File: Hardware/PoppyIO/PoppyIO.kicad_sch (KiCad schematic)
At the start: 0 parts

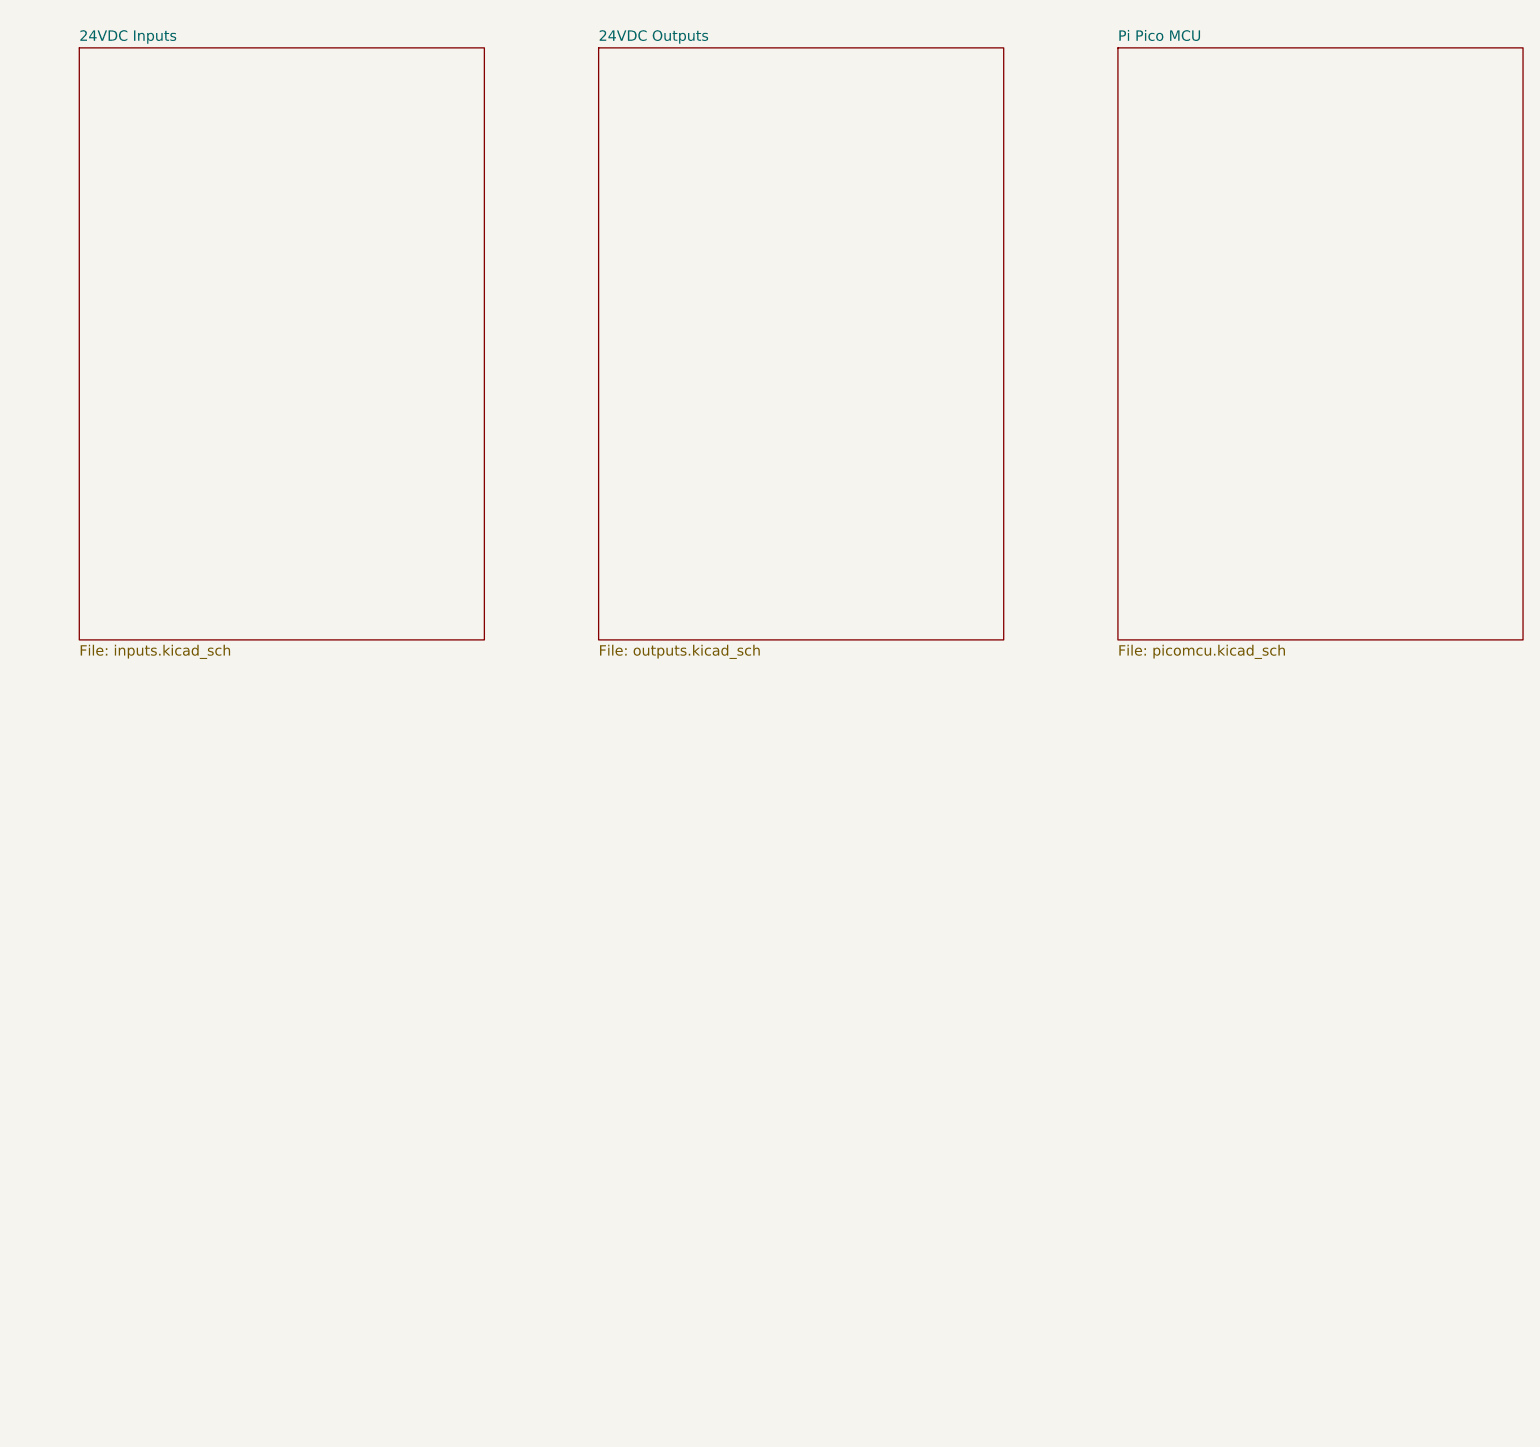
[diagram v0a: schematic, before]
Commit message: hw: io: Updates
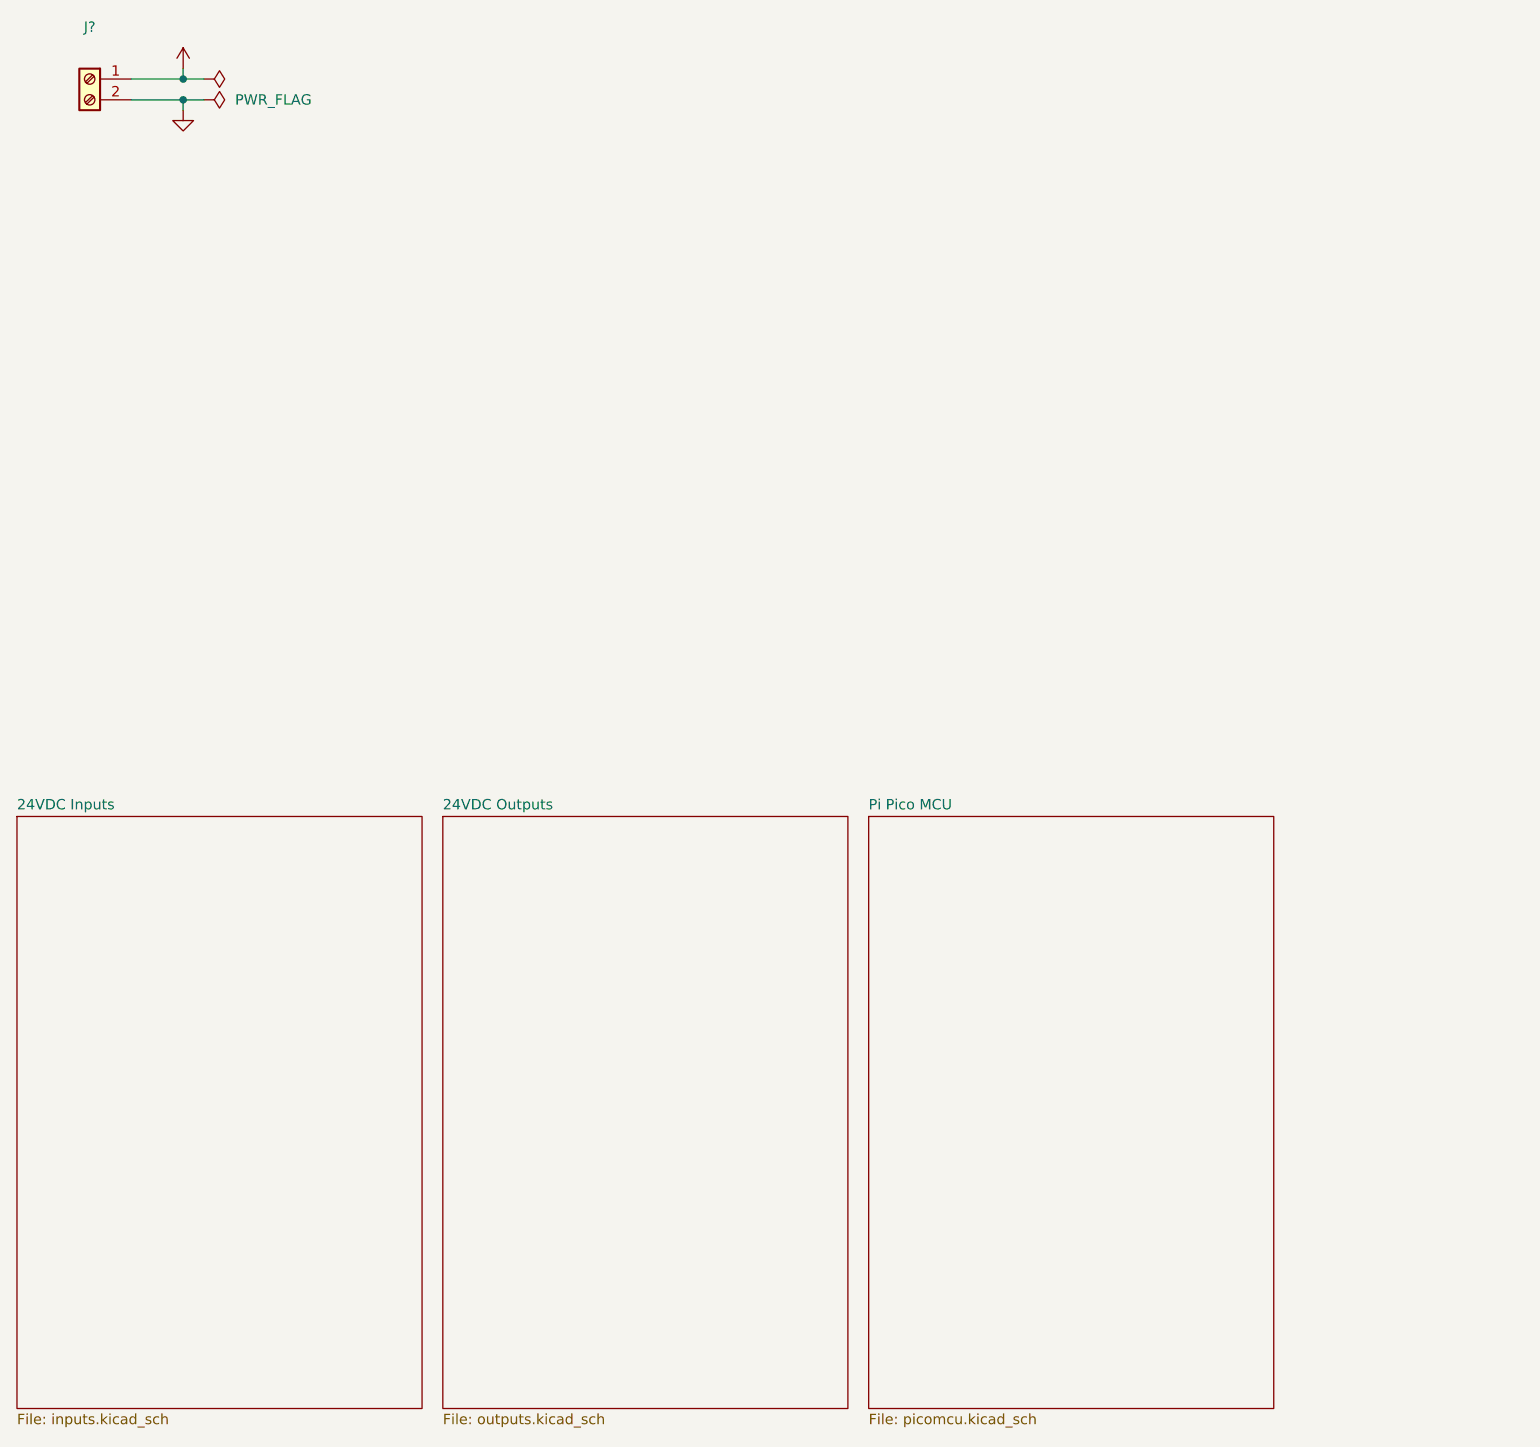
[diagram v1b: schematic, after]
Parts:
- added J?: (no value), symbol Connector:Screw_Terminal_01x02
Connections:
- new net +5V: J?.1 (Pin_1)
- new net GND: J?.2 (Pin_2)

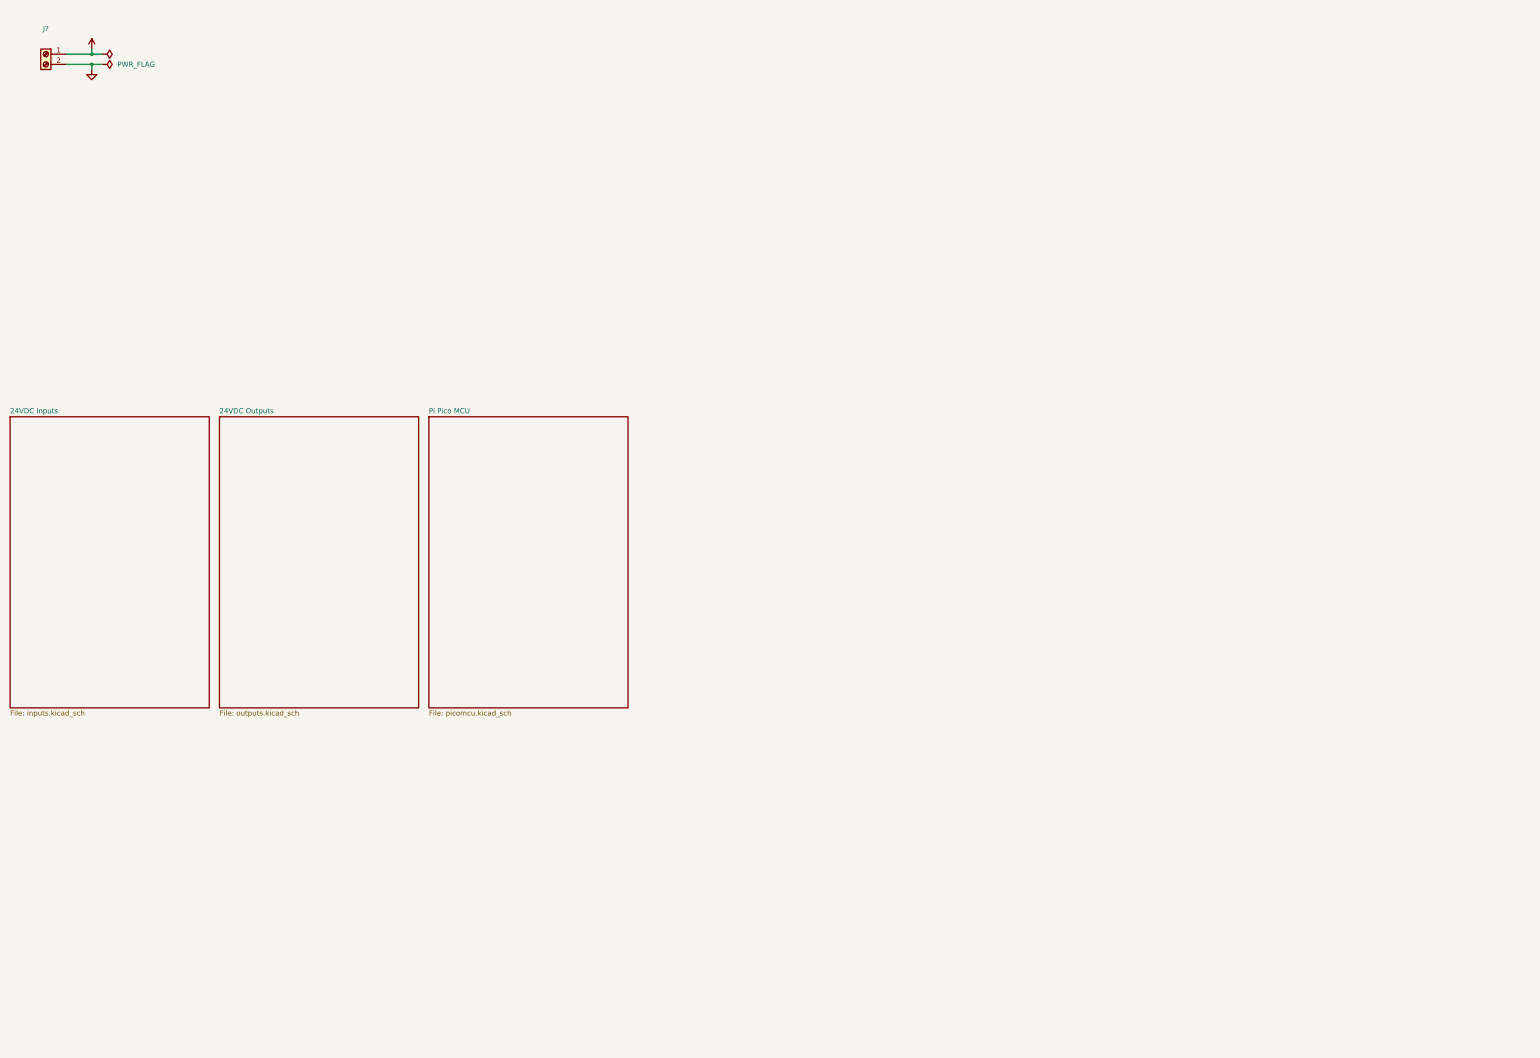
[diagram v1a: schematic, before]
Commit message: hw: io: Single sheet
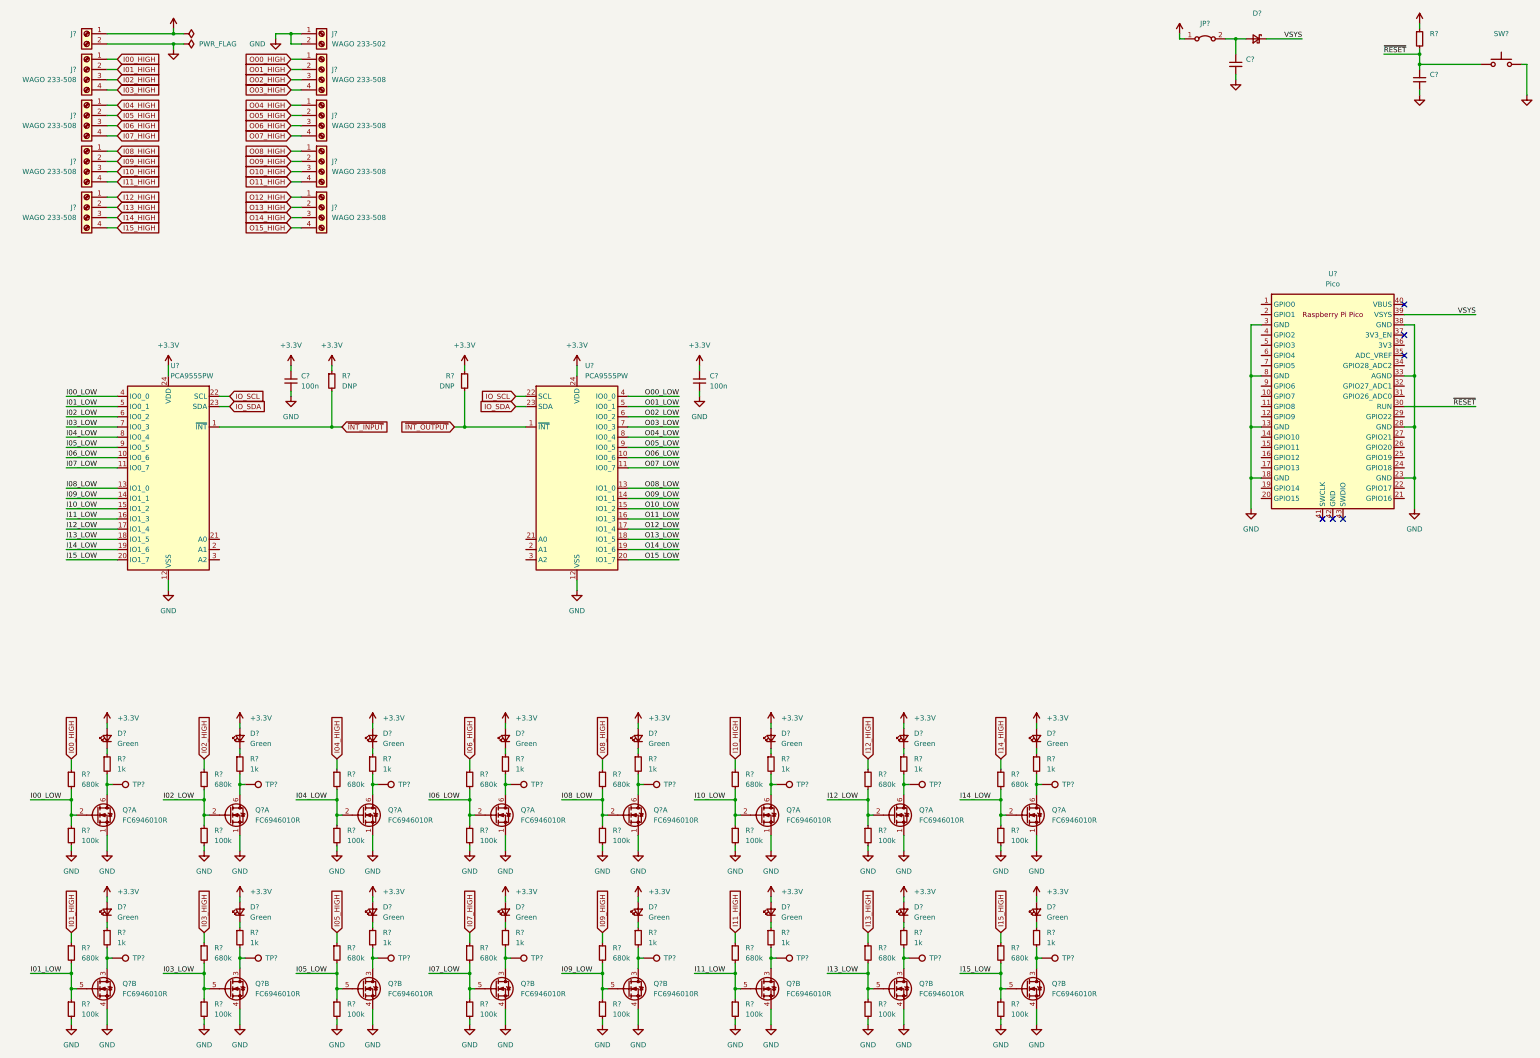
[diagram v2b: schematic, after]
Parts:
- added C? (x2): (no value), symbol Device:C_Small
- added C? (x2): 100n, symbol Device:C_Small
- added D? (x16): Green, symbol Device:LED_Small
- added D?: (no value), symbol Device:D_Schottky_Small
- added J? (x8): WAGO 233-508, symbol Connector:Screw_Terminal_01x04
- added J?: WAGO 233-502, symbol Connector:Screw_Terminal_01x02
- added JP?: ~, symbol Jumper:Jumper_2_Bridged
- added Q? (x16): FC6946010R, symbol Device:Q_Dual_NMOS_S1G1D2S2G2D1
- added R? (x16): 680k, symbol Device:R_Small
- added R? (x16): 1k, symbol Device:R_Small
- added R? (x16): 100k, symbol Device:R_Small
- added R? (x2): DNP, symbol Device:R_Small
- added R?: (no value), symbol Device:R_Small
- added SW?: (no value), symbol Switch:SW_Push
- added TP? (x16): TestPoint, symbol Connector:TestPoint
- added U?: Pico, RPi_Pico:RPi_Pico_SMD_TH, symbol RPi_Pico:Pico
- added U? (x2): PCA9555PW, Package_SO:TSSOP-24_4.4x7.8mm_P0.65mm, symbol Interface_Expansion:PCA9555PW
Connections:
- net +5V: now also JP?.1 (A)
- net GND: now also C?.2, C?.2, C?.2, C?.2, J?.1 (Pin_1), J?.2 (Pin_2), Q?.1 (S), Q?.1 (S), Q?.1 (S), Q?.1 (S), Q?.1 (S), Q?.1 (S), Q?.1 (S), Q?.1 (S), Q?.4 (S), Q?.4 (S), Q?.4 (S), Q?.4 (S), Q?.4 (S), Q?.4 (S), Q?.4 (S), Q?.4 (S), R?.2, R?.2, R?.2, R?.2, R?.2, R?.2, R?.2, R?.2, R?.2, R?.2, R?.2, R?.2, R?.2, R?.2, R?.2, R?.2, SW?.2, U?.12 (VSS), U?.12 (VSS), U?.13 (GND), U?.18 (GND), U?.23 (GND), U?.28 (GND), U?.3 (GND), U?.33 (AGND), U?.38 (GND), U?.8 (GND)
- new net: D?.1 (K), R?.1 (x16)
- new net: Q?.3 (D), R?.2, TP?.1 (x8)
- new net: Q?.6 (D), R?.2, TP?.1 (x8)
- new net: C?.1, D?.2 (A), JP?.2 (B)
- new net +3V3: C?.1, C?.1, D?.2 (A), D?.2 (A), D?.2 (A), D?.2 (A), D?.2 (A), D?.2 (A), D?.2 (A), D?.2 (A), D?.2 (A), D?.2 (A), D?.2 (A), D?.2 (A), D?.2 (A), D?.2 (A), D?.2 (A), D?.2 (A), R?.1, R?.1, R?.1, U?.24 (VDD), U?.24 (VDD)
- new net I00_HIGH: J?.1 (Pin_1), R?.1
- new net I00_LOW: Q?.2 (G), R?.1, R?.2, U?.4 (IO0_0)
- new net I01_HIGH: J?.2 (Pin_2), R?.1
- new net I01_LOW: Q?.5 (G), R?.1, R?.2, U?.5 (IO0_1)
- new net I02_HIGH: J?.3 (Pin_3), R?.1
- new net I02_LOW: Q?.2 (G), R?.1, R?.2, U?.6 (IO0_2)
- new net I03_HIGH: J?.4 (Pin_4), R?.1
- new net I03_LOW: Q?.5 (G), R?.1, R?.2, U?.7 (IO0_3)
- new net I04_HIGH: J?.1 (Pin_1), R?.1
- new net I04_LOW: Q?.2 (G), R?.1, R?.2, U?.8 (IO0_4)
- new net I05_HIGH: J?.2 (Pin_2), R?.1
- new net I05_LOW: Q?.5 (G), R?.1, R?.2, U?.9 (IO0_5)
- new net I06_HIGH: J?.3 (Pin_3), R?.1
- new net I06_LOW: Q?.2 (G), R?.1, R?.2, U?.10 (IO0_6)
- new net I07_HIGH: J?.4 (Pin_4), R?.1
- new net I07_LOW: Q?.5 (G), R?.1, R?.2, U?.11 (IO0_7)
- new net I08_HIGH: J?.1 (Pin_1), R?.1
- new net I08_LOW: Q?.2 (G), R?.1, R?.2, U?.13 (IO1_0)
- new net I09_HIGH: J?.2 (Pin_2), R?.1
- new net I09_LOW: Q?.5 (G), R?.1, R?.2, U?.14 (IO1_1)
- new net I10_HIGH: J?.3 (Pin_3), R?.1
- new net I10_LOW: Q?.2 (G), R?.1, R?.2, U?.15 (IO1_2)
- new net I11_HIGH: J?.4 (Pin_4), R?.1
- new net I11_LOW: Q?.5 (G), R?.1, R?.2, U?.16 (IO1_3)
- new net I12_HIGH: J?.1 (Pin_1), R?.1
- new net I12_LOW: Q?.2 (G), R?.1, R?.2, U?.17 (IO1_4)
- new net I13_HIGH: J?.2 (Pin_2), R?.1
- new net I13_LOW: Q?.5 (G), R?.1, R?.2, U?.18 (IO1_5)
- new net I14_HIGH: J?.3 (Pin_3), R?.1
- new net I14_LOW: Q?.2 (G), R?.1, R?.2, U?.19 (IO1_6)
- new net I15_HIGH: J?.4 (Pin_4), R?.1
- new net I15_LOW: Q?.5 (G), R?.1, R?.2, U?.20 (IO1_7)
- new net IO_SCL: U?.22 (SCL), U?.22 (SCL)
- new net IO_SDA: U?.23 (SDA), U?.23 (SDA)
- new net O00_HIGH: J?.1 (Pin_1)
- new net O00_LOW: U?.4 (IO0_0)
- new net O01_HIGH: J?.2 (Pin_2)
- new net O01_LOW: U?.5 (IO0_1)
- new net O02_HIGH: J?.3 (Pin_3)
- new net O02_LOW: U?.6 (IO0_2)
- new net O03_HIGH: J?.4 (Pin_4)
- new net O03_LOW: U?.7 (IO0_3)
- new net O04_HIGH: J?.1 (Pin_1)
- new net O04_LOW: U?.8 (IO0_4)
- new net O05_HIGH: J?.2 (Pin_2)
- new net O05_LOW: U?.9 (IO0_5)
- new net O06_HIGH: J?.3 (Pin_3)
- new net O06_LOW: U?.10 (IO0_6)
- new net O07_HIGH: J?.4 (Pin_4)
- new net O07_LOW: U?.11 (IO0_7)
- new net O08_HIGH: J?.1 (Pin_1)
- new net O08_LOW: U?.13 (IO1_0)
- new net O09_HIGH: J?.2 (Pin_2)
- new net O09_LOW: U?.14 (IO1_1)
- new net O10_HIGH: J?.3 (Pin_3)
- new net O10_LOW: U?.15 (IO1_2)
- new net O11_HIGH: J?.4 (Pin_4)
- new net O11_LOW: U?.16 (IO1_3)
- new net O12_HIGH: J?.1 (Pin_1)
- new net O12_LOW: U?.17 (IO1_4)
- new net O13_HIGH: J?.2 (Pin_2)
- new net O13_LOW: U?.18 (IO1_5)
- new net O14_HIGH: J?.3 (Pin_3)
- new net O14_LOW: U?.19 (IO1_6)
- new net O15_HIGH: J?.4 (Pin_4)
- new net O15_LOW: U?.20 (IO1_7)
- new net VSYS: D?.1 (K), U?.39 (VSYS)
- new net ~{INT_INPUT}: R?.2, U?.1 (~{INT})
- new net ~{INT_OUTPUT}: R?.2, U?.1 (~{INT})
- new net ~{RESET}: C?.1, R?.2, SW?.1, U?.30 (RUN)
- no-connect marks 0 -> 6
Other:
- removed sheet 24VDC Inputs
- removed sheet 24VDC Outputs
- removed sheet Pi Pico MCU
- moved on the sheet: J?
